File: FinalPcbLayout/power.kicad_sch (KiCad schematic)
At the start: 17 parts, among them J3 Barrel_Jack, Q4 PMOS, U3 TPS63070RNMR, U4 LDI1117-3.3H

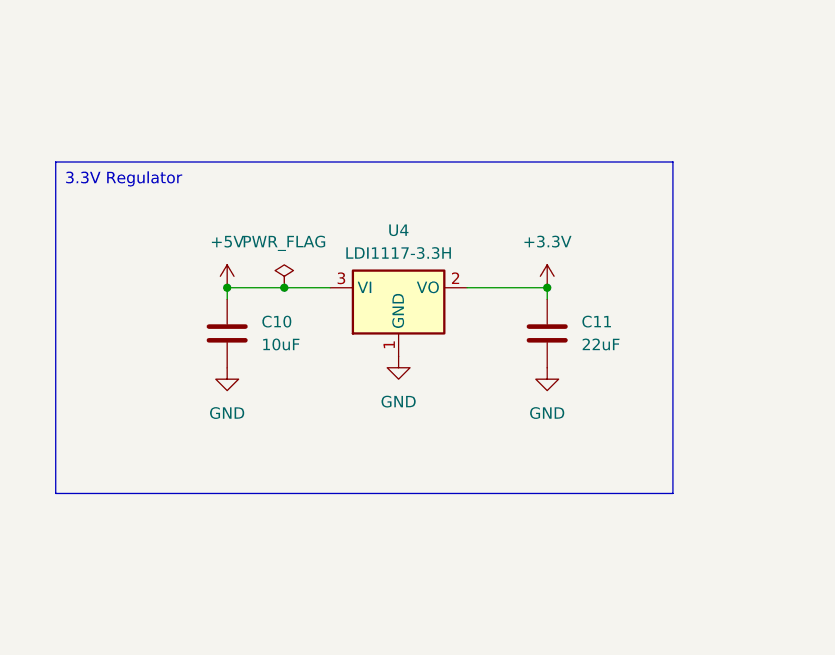
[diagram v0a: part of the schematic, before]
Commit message: Working on USB to UART
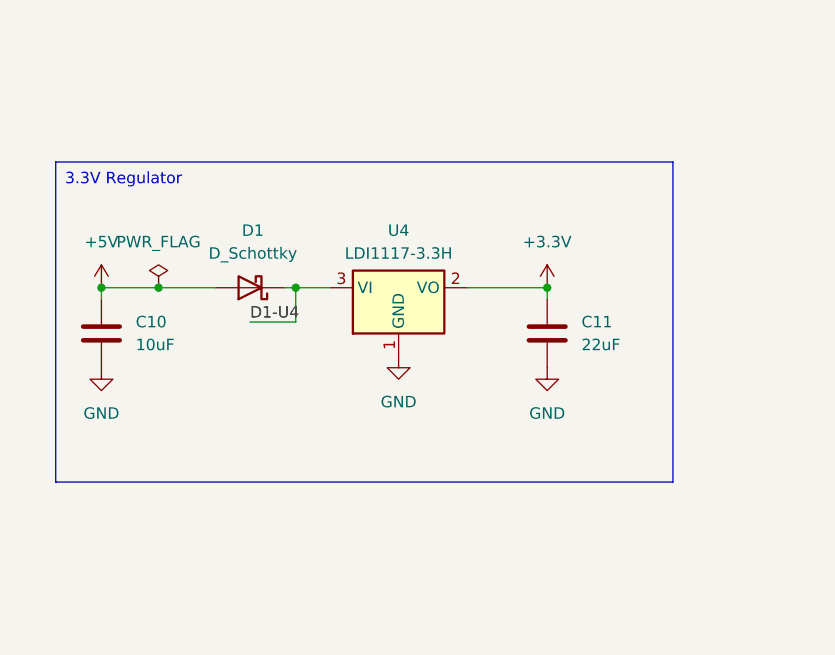
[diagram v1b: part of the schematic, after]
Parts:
- added D1: D_Schottky, Diode_SMD:D_SMA, symbol Device:D_Schottky
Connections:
- net +5V: now also D1.2 (A); no longer U4.3 (VI)
- new net D1-U4: D1.1 (K), U4.3 (VI)
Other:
- moved on the sheet: C10
